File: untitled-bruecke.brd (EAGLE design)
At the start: 100 x 80 mm, 7 parts

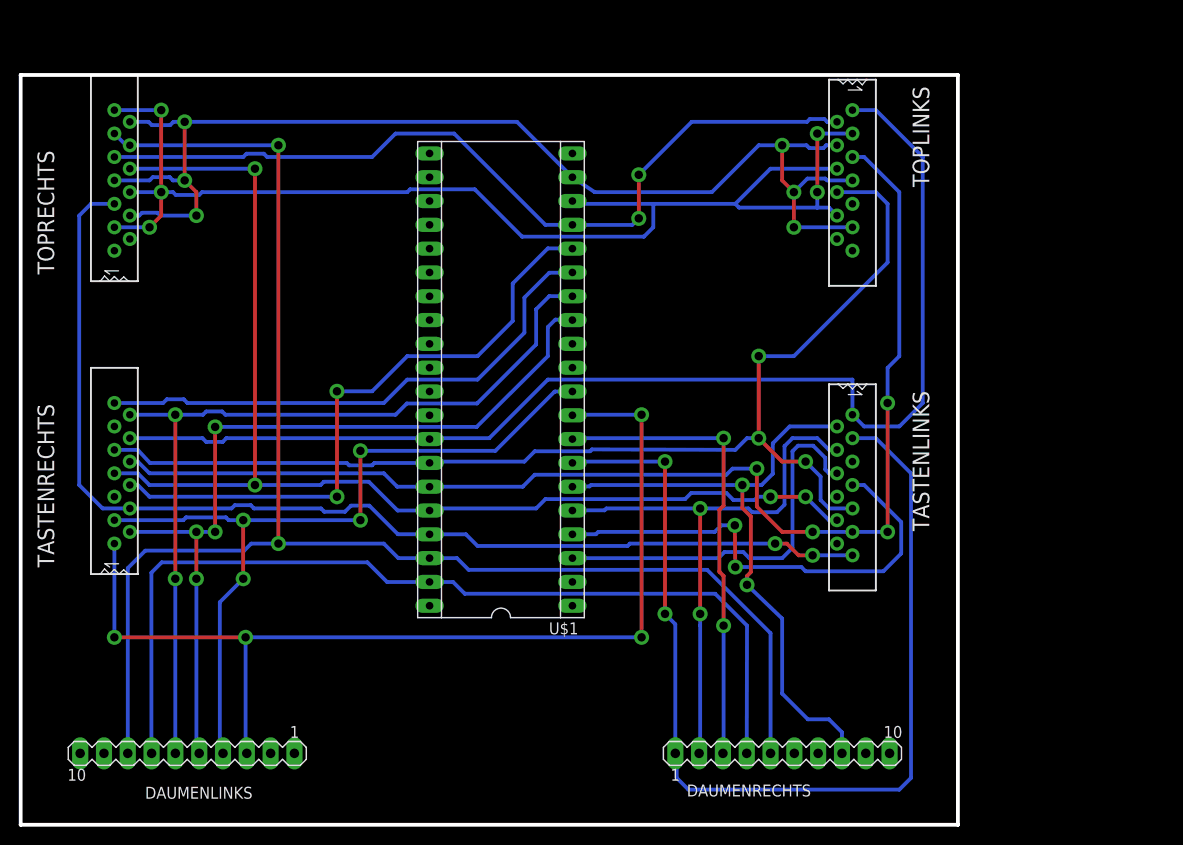
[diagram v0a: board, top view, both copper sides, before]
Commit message: Layout fertiggestellt fürs PCB
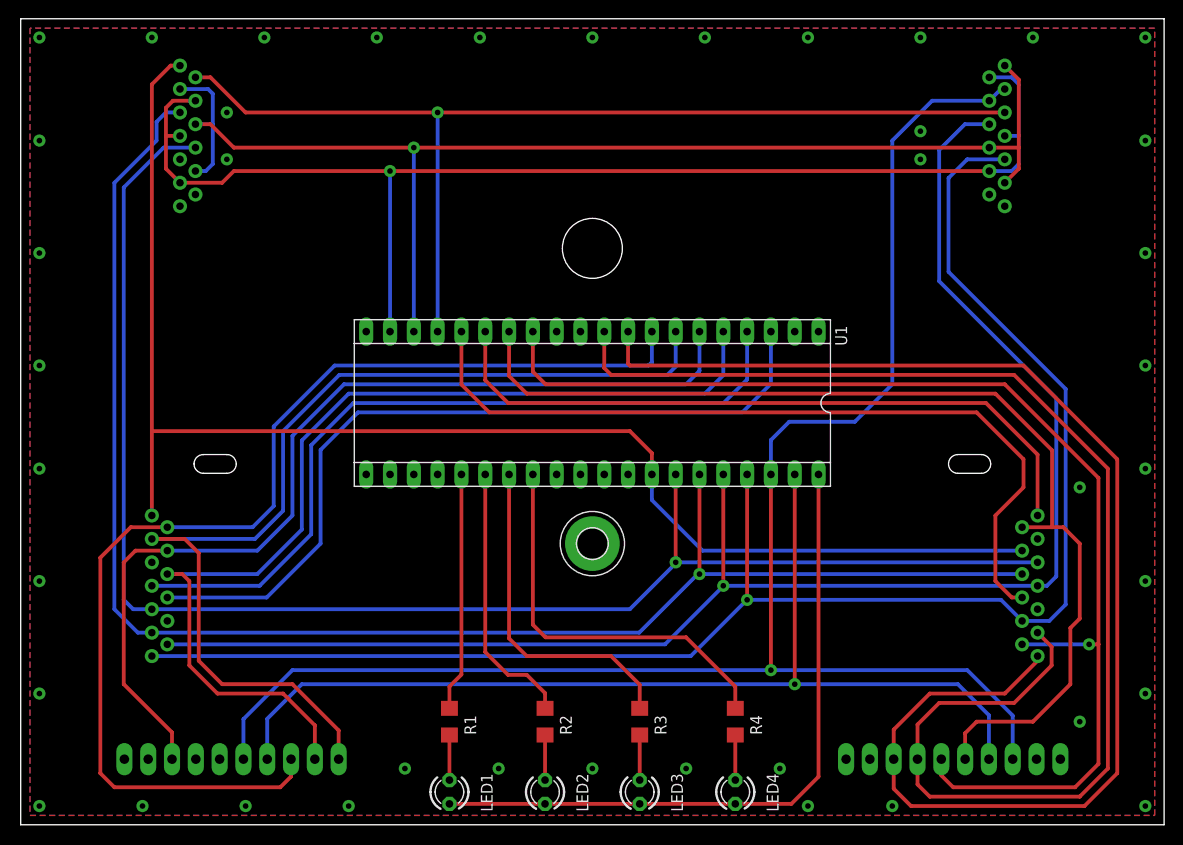
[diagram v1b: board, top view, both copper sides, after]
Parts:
- removed U$1: C-TEENSY++, teensypp:TEENSY++
- added E$1: (no value), holes:3,2-PAD
- added LED1, LED2, LED3, LED4: (no value), led:LED3MM
- added R1, R2, R3, R4: (no value), rcl:R1206
- added U1: C-TEENSY++, teensypp:TEENSY++
- moved TASTENRECHTS 99.2 mm to (108.5, 25.5), flipped to the bottom
- moved TOPRECHTS 95.1 mm to (105.0, 73.5), flipped to the bottom
- moved DAUMENLINKS 81.7 mm to (99.5, 7.00), flipped to the bottom
- moved TASTENLINKS 75.5 mm to (14.0, 25.5), flipped to the bottom
- moved TOPLINKS 71.9 mm to (17.0, 73.5), flipped to the bottom
- moved DAUMENRECHTS 58.8 mm to (22.5, 7.00), flipped to the bottom
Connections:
- removed net VCC: U$1.+5V
- new net N$10: R4.2, U1.F0
- new net N$11: LED1.A, LED2.A, LED3.A, LED4.A, U1.+5V
- new net N$14: LED4.K, R4.1
- new net N$15: LED3.K, R3.1
- new net N$16: LED2.K, R2.1
- new net N$17: LED1.K, R1.1
- new net N$7: R1.2, U1.F3
- new net N$8: R2.2, U1.F2
- new net N$9: R3.2, U1.F1
- net B0: now also U1.B0; no longer U$1.B0
- net B1: now also U1.B1; no longer U$1.B1
- net B2: now also U1.B2; no longer U$1.B2
- net B3: now also TASTENLINKS.P$12, U1.B3; no longer TASTENLINKS.P$10, U$1.B3
- net B4: now also U1.B4; no longer U$1.B4
- net B5: now also U1.B5; no longer U$1.B5
- net B6: now also U1.B6; no longer U$1.B6
- net C0: now also U1.C0; no longer U$1.C0
- net C1: now also U1.C1; no longer U$1.C1
- net C2: now also U1.C2; no longer U$1.C2
- net C3: now also U1.C3; no longer U$1.C3
- net C4: now also U1.C4; no longer U$1.C4
- net C5: now also U1.C5; no longer U$1.C5
- net C6: now also U1.C6; no longer U$1.C6
- net D0: now also TASTENLINKS.P$8, U1.D0; no longer TASTENLINKS.P$6, U$1.D0
- net D1: now also U1.D1; no longer U$1.D1
- net D2: now also TASTENLINKS.P$6, U1.D2; no longer TASTENLINKS.P$4, U$1.D2
- net D3: now also TASTENLINKS.P$4, U1.D3; no longer TASTENLINKS.P$2, U$1.D3
- net D4: now also U1.D4; no longer U$1.D4
- net D5: now also TASTENLINKS.P$2, U1.D5; no longer U$1.D5
- net D6: now also U1.D6; no longer U$1.D6
- net D7: now also U1.D7; no longer U$1.D7
- net GND: now also U1.GRND1; no longer U$1.GRND1
- net N$1: now also U1.GND; no longer U$1.GND
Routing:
- net N$11: track 0.00 -> 72.8 mm
- net D5: track 50.6 -> 122.0 mm, vias 2 -> 0
- net D7: track 85.2 -> 143.6 mm, vias 4 -> 0
- net B4: track 119.7 -> 172.5 mm, vias 2 -> 1
- net D2: track 62.1 -> 109.6 mm, vias 2 -> 0
- net D0: track 41.7 -> 85.3 mm
- net N$10: track 0.00 -> 42.7 mm
- net C0: track 88.7 -> 128.0 mm, vias 4 -> 1
- net B1: track 124.1 -> 162.9 mm, vias 3 -> 1
- net B3: track 128.3 -> 166.9 mm, vias 4 -> 1
- net B2: track 131.2 -> 167.9 mm, vias 4 -> 1
- net N$9: track 0.00 -> 36.0 mm
- net D3: track 67.5 -> 102.2 mm, vias 2 -> 0
- net D6: track 111.4 -> 144.6 mm, vias 4 -> 0
- net D1: track 51.0 -> 83.3 mm, vias 2 -> 0
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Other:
- board size 100 x 80 mm -> 122 x 86 mm
- board text added: "28.02.2013"
- board text added: "CAPS"
- board text added: "KEYPAD"
- board text added: "M. Stapelberg / V. Wunsch"
- board text added: "NUM"
- board text added: "SCR"
- board text added: "Teensy++ Kinesis controller"
